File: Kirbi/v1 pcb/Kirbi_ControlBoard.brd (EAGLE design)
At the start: 66 x 56 mm, 71 parts, among them U1 PCA9306_LSSOP, U2 TEENSY_3.6_DIL, U5 LM393-8-SOIC, U6 AP2114H-1.8TRG1, U7 AP2114H-3.3TRG1

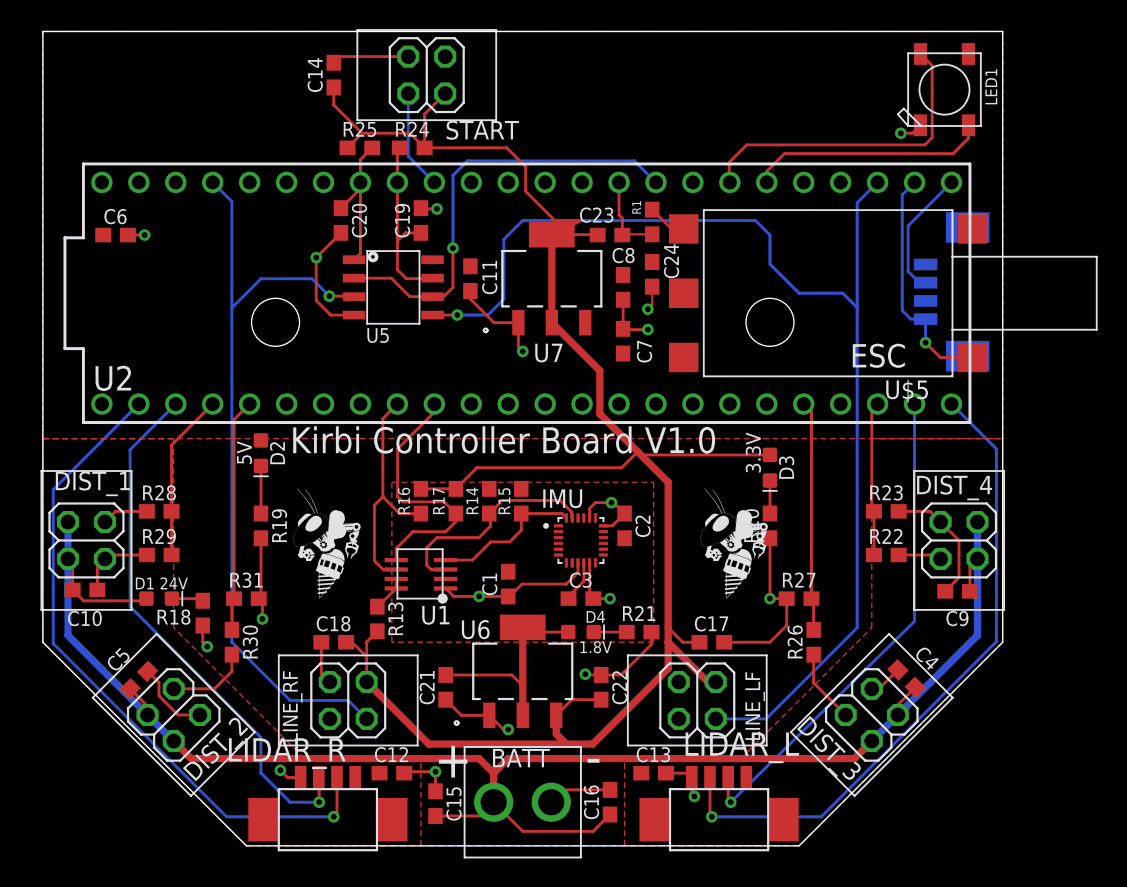
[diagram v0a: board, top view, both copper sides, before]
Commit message: Moved LEDs and NeoPixel to bottom
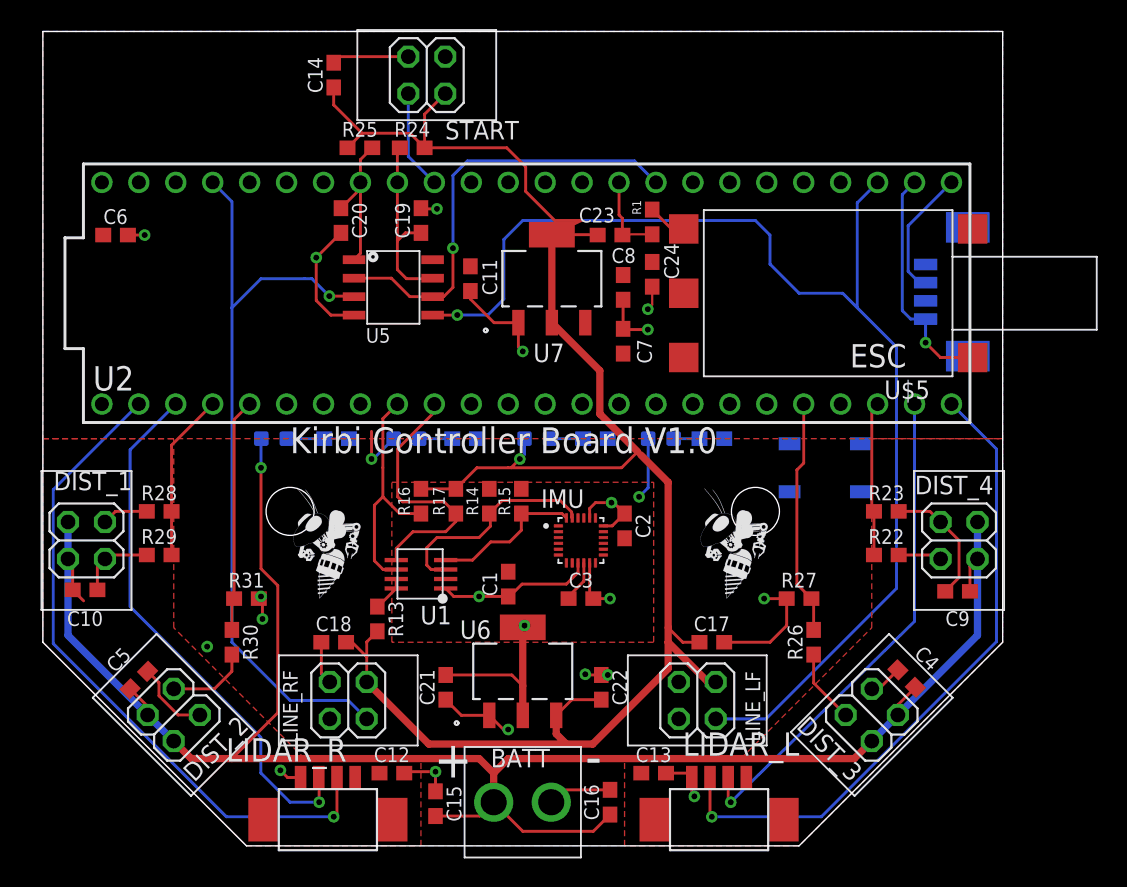
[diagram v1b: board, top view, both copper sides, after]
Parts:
- moved LED1 27.3 mm to (39.8, 26.0), flipped to the bottom, turned to 180 degrees
- moved D3 16.1 mm to (20.0, 28.0), flipped to the bottom, turned to 180 degrees
- moved R19 15.2 mm to (15.0, 28.0), flipped to the bottom, turned to 180 degrees
- moved R18 15.1 mm to (6.20, 28.0), flipped to the bottom, turned to 180 degrees
- moved D4 14.4 mm to (28.5, 28.0), flipped to the bottom, turned to 180 degrees
- moved R21 14.2 mm to (32.0, 28.0), flipped to the bottom, turned to 180 degrees
- moved D1 13.5 mm to (1.90, 28.0), flipped to the bottom, turned to 180 degrees
- moved R20 13.4 mm to (24.0, 28.0), flipped to the bottom, turned to 180 degrees
- moved D2 10.0 mm to (11.0, 28.0), flipped to the bottom, turned to 180 degrees
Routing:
- net NEO_DO: track 22.1 -> 0.06 mm
- net 24V: track 116.5 -> 135.9 mm, vias 0 -> 1
- net NEO_DI: track 16.5 -> 0.00 mm
- net GND: track 123.4 -> 107.9 mm, vias 18 -> 19
- net +3.3V: track 135.0 -> 127.9 mm, vias 0 -> 1
- net +5V: track 0.00 -> 4.00 mm, vias 0 -> 1
- net LINE_LF: track 81.5 -> 83.7 mm
- net N$6: track 2.19 -> 4.27 mm
- net 1.8V: track 14.9 -> 16.1 mm, vias 0 -> 2
- net N$1: track 3.27 -> 2.27 mm
- net N$10: track 2.27 -> 1.77 mm

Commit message: Moved NeoPixel to the center
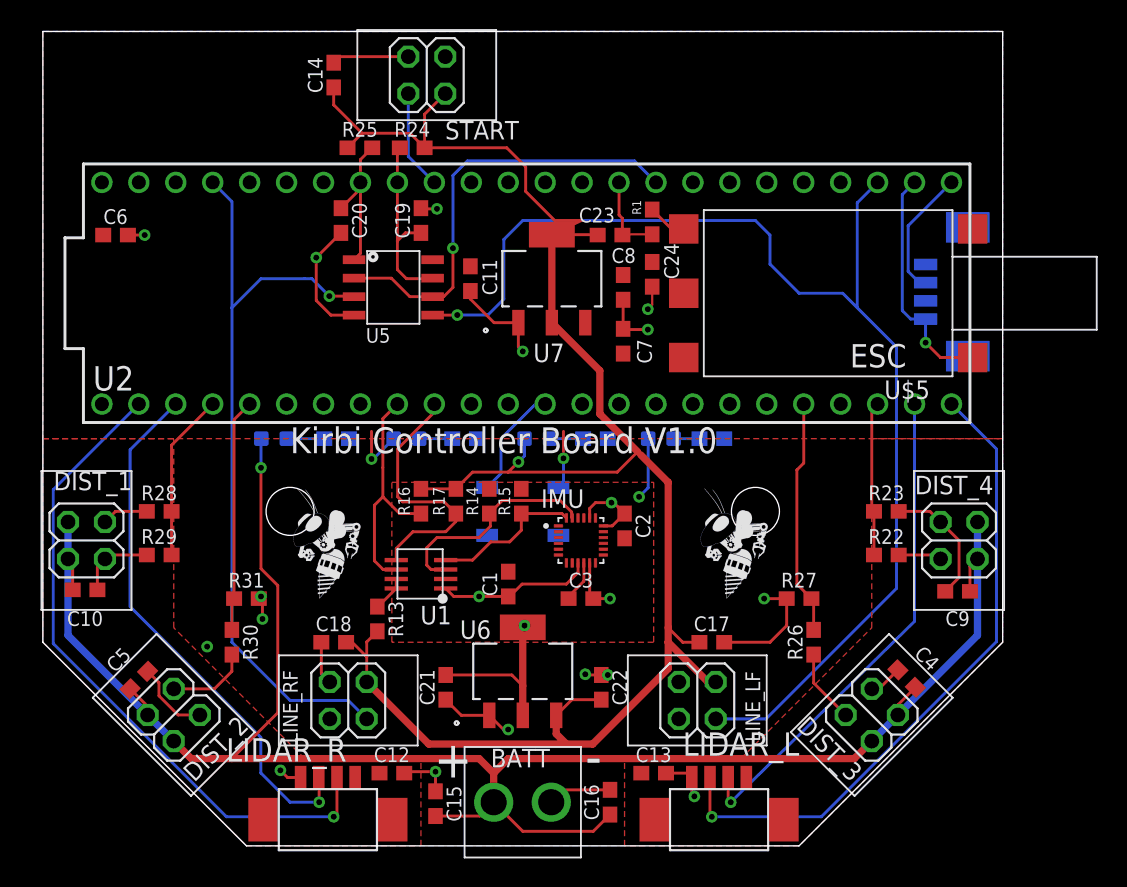
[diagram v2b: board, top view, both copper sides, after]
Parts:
- moved LED1 21.0 mm to (19.0, 23.0)
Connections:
- net NEO_DI: now also U2.11; no longer U2.38/A19
- net NEO_DO: no longer U2.39/A20
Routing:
- net NEO_DI: track 0.00 -> 7.77 mm
- net +5V: track 4.00 -> 8.00 mm, vias 1 -> 2
- net N$6: track 4.27 -> 2.57 mm
- net 24V: track 135.9 -> 134.9 mm
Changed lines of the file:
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@@
 <attribute name="VALUE" x="28" y="4.238" size="0.6096" layer="27" font="vector" ratio="20" align="top-center"/>
 </element>
-<element name="LED1" library="adafruit" library_urn="urn:adsk.eagle:library:420" package="WS2812B" package3d_urn="urn:adsk.eagle:package:6240942/1" value="WS2812B5050" x="39.8" y="26" smashed="yes" rot="MR180">
-<attribute name="NAME" x="36.2925" y="27.8125" size="0.8128" layer="26" ratio="10" rot="MR270"/>
+<element name="LED1" library="adafruit" library_urn="urn:adsk.eagle:library:420" package="WS2812B" package3d_urn="urn:adsk.eagle:package:6240942/1" value="WS2812B5050" x="19" y="23" smashed="yes" rot="MR180">
+<attribute name="NAME" x="15.4925" y="24.8125" size="0.8128" layer="26" ratio="10" rot="MR270"/>
 </element>
 <element name="ESC" library="Kirbi_ControlBoard" package="MOLEX_1.25MM_4PIN_SMT" value="MOLEX_1.25MM_4PIN_SMT" x="49.6" y="38.1" smashed="yes" rot="MR270">
@@
 <wire x1="12" y1="43.85" x2="12.05" y2="43.8" width="0.2" layer="1"/>
 <wire x1="1" y1="17.15" x2="0.85" y2="17" width="0.2" layer="1"/>
-<wire x1="25.030721875" y1="27.969278125" x2="24.85" y2="28" width="0.2" layer="16"/>
 <contactref element="LED1" pad="3-GND"/>
 <wire x1="6.5" y1="42.15" x2="4.8" y2="40.45" width="0.2" layer="1"/>
@@
 <via x="8.6" y="26.6" extent="1-16" drill="0.4"/>
 <wire x1="8.6" y1="26.6" x2="8.6" y2="28.5" width="0.2" layer="1"/>
-<wire x1="30.07" y1="33.58" x2="42.25" y2="27.65" width="0" layer="19" extent="1-16"/>
+<wire x1="21.45" y1="24.65" x2="21.8" y2="25" width="0.2" layer="16"/>
+<wire x1="21.8" y1="25" x2="21.8" y2="26.6444" width="0.2" layer="16"/>
+<via x="21.8" y="26.6444" extent="1-16" drill="0.4"/>
+<wire x1="21.8" y1="26.6444" x2="21.8" y2="28.5" width="0.2" layer="1"/>
 </signal>
 <signal name="+3.3V">
@@
 <contactref element="R17" pad="2"/>
 <contactref element="R13" pad="2"/>
-<wire x1="14.4" y1="24.55" x2="15.85" y2="26" width="0.2" layer="1"/>
-<wire x1="25.8" y1="26" x2="26.9" y2="27.1" width="0.2" layer="1"/>
-<wire x1="15.85" y1="26" x2="18" y2="26" width="0.2" layer="1"/>
-<wire x1="18.2" y1="26" x2="25.8" y2="26" width="0.2" layer="1"/>
+<wire x1="14.4" y1="24.55" x2="15.55" y2="25.7" width="0.2" layer="1"/>
+<wire x1="25.5" y1="25.7" x2="26.9" y2="27.1" width="0.2" layer="1"/>
+<wire x1="15.55" y1="25.7" x2="18" y2="25.7" width="0.2" layer="1"/>
+<wire x1="18" y1="25.7" x2="25.5" y2="25.7" width="0.2" layer="1"/>
 <wire x1="12" y1="24.55" x2="14.4" y2="24.55" width="0.2" layer="1"/>
 <contactref element="LINE_LF" pad="1"/>
@@
 <wire x1="31.15" y1="14" x2="30" y2="14" width="0.2" layer="1"/>
 <wire x1="30" y1="14" x2="29" y2="15" width="0.2" layer="1"/>
-<wire x1="19.123" y1="28" x2="19.123" y2="26.923" width="0.2" layer="16"/>
-<wire x1="19.123" y1="26.923" x2="18.8" y2="26.6" width="0.2" layer="16"/>
-<via x="18.8" y="26.6" extent="1-16" drill="0.4"/>
-<wire x1="18.8" y1="26.6" x2="18.2" y2="26" width="0.2" layer="1"/>
-<wire x1="18.2" y1="26" x2="18" y2="26" width="0.2" layer="1"/>
+<wire x1="19.123" y1="28" x2="19.123" y2="26.823" width="0.2" layer="16"/>
+<wire x1="19.123" y1="26.823" x2="18.7" y2="26.4" width="0.2" layer="16"/>
+<via x="18.7" y="26.4" extent="1-16" drill="0.4"/>
+<wire x1="18.7" y1="26.4" x2="18" y2="25.7" width="0.2" layer="1"/>
 <wire x1="27.123" y1="26.877" x2="19.123" y2="28" width="0" layer="19" extent="1-16"/>
 </signal>
@@
 <wire x1="-12.27" y1="19.73" x2="-12.27" y2="22.27" width="0.5" layer="16"/>
 <wire x1="-12.27" y1="19.73" x2="-11.95" y2="19.41" width="0.2" layer="1"/>
-<wire x1="-11.95" y1="17.6" x2="-11.1976" y2="16.8476" width="0.2" layer="1"/>
 <wire x1="50.27" y1="14.47395" x2="44.79605" y2="9" width="0.5" layer="16"/>
 <wire x1="50.27" y1="22.27" x2="50.27" y2="19.73" width="0.5" layer="16"/>
@@
 <contactref element="D1" pad="C"/>
 <contactref element="R18" pad="1"/>
-<wire x1="7.05" y1="28" x2="5.35" y2="28" width="0.1524" layer="16"/>
 <wire x1="2.777" y1="28" x2="5.35" y2="28" width="0.2" layer="16"/>
 </signal>
@@
 <signal name="NEO_DO">
 <contactref element="LED1" pad="2-DOUT"/>
-<contactref element="U2" pad="39/A20"/>
-<wire x1="33.24" y1="45.62" x2="33.2" y2="45.66" width="0.2" layer="1"/>
-<wire x1="42.25" y1="24.35" x2="33.24" y2="45.62" width="0" layer="19" extent="16-16"/>
 </signal>
 <signal name="NEO_DI">
 <contactref element="LED1" pad="4-DIN"/>
-<contactref element="U2" pad="38/A19"/>
-<wire x1="37.35" y1="27.65" x2="35.78" y2="45.62" width="0" layer="19" extent="16-16"/>
+<contactref element="U2" pad="11"/>
+<wire x1="16.55" y1="24.65" x2="17.5" y2="25.6" width="0.2" layer="16"/>
+<wire x1="17.5" y1="25.6" x2="17.5" y2="28" width="0.2" layer="16"/>
+<wire x1="17.5" y1="28" x2="19.88" y2="30.38" width="0.2" layer="16"/>
+<wire x1="19.88" y1="30.38" x2="20.54" y2="30.38" width="0.2" layer="16"/>
 </signal>
 <signal name="N$8">
